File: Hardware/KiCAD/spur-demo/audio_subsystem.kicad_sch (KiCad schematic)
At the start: 25 parts, among them U3 MAX98357A, U4 LM393

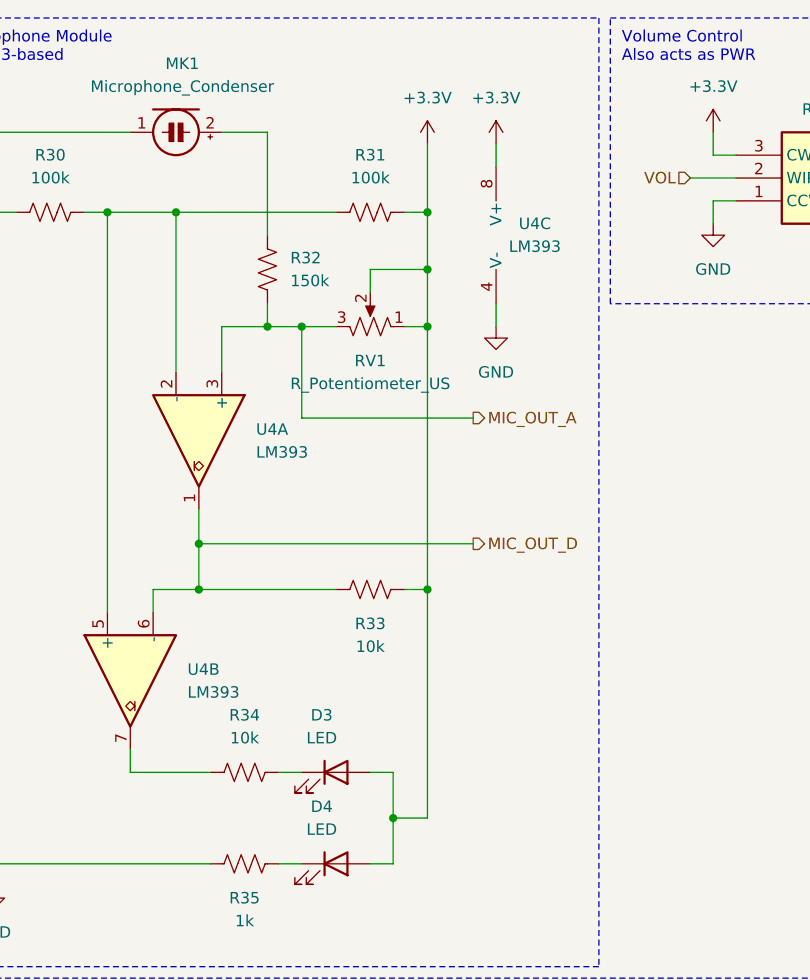
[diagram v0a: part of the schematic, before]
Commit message: fix: give mic level setpoint potentiometer a name
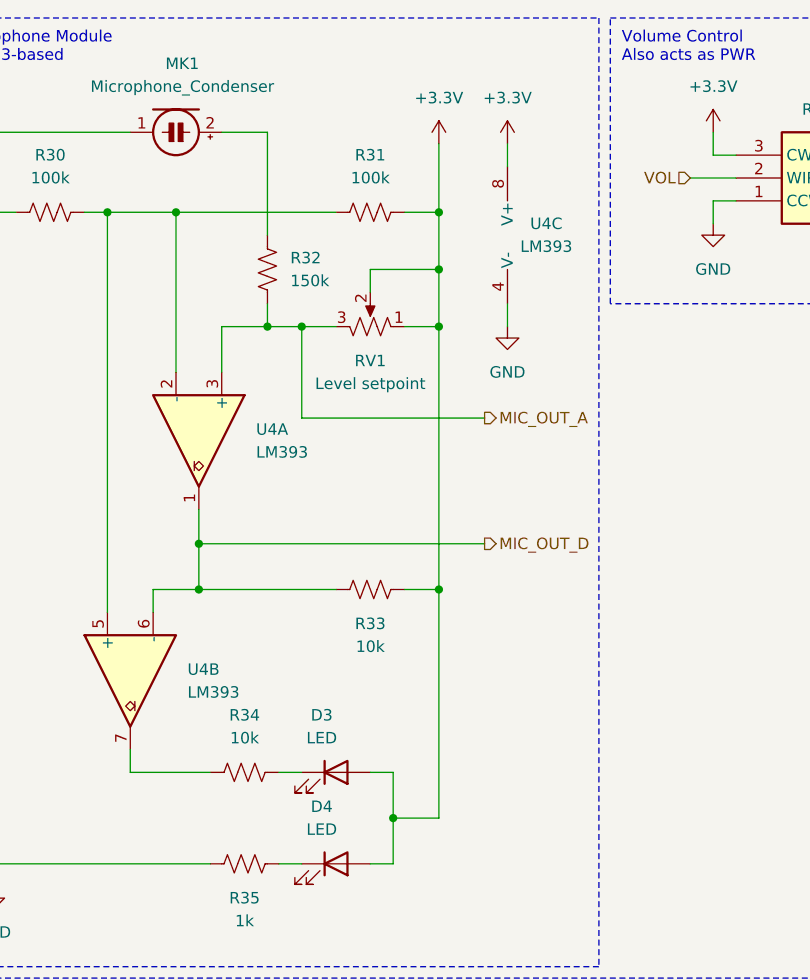
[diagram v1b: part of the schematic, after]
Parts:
- RV1: value R_Potentiometer_US -> Level setpoint
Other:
- moved on the sheet: U4C

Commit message: feat: begin footprint assignment, unify +3.3V PWRREFs
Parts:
- D3, D4: footprint (none) -> LED_SMD:LED_0603_1608Metric_Pad1.05x0.95mm_HandSolder
- LS1: footprint (none) -> Connector_JST:JST_XH_S2B-XH-A_1x02_P2.50mm_Horizontal
- MK1: footprint (none) -> Sensor_Audio:POM-2244P-C3310-2-R
- R13, R14, R28, R29, R30, R31, R32, R33, R34, R35, R37: footprint (none) -> Resistor_SMD:R_0603_1608Metric
- RV1: footprint (none) -> Potentiometer_SMD:Potentiometer_Bourns_3214W_Vertical
- U4: footprint (none) -> Package_SO:VSSOP-8_3x3mm_P0.65mm
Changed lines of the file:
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@@
 			)
 		)
-		(property "Footprint" ""
+		(property "Footprint" "LED_SMD:LED_0603_1608Metric_Pad1.05x0.95mm_HandSolder"
 			(at 57.15 107.95 0)
 			(effects
@@
 			)
 		)
-		(property "Footprint" ""
+		(property "Footprint" "LED_SMD:LED_0603_1608Metric_Pad1.05x0.95mm_HandSolder"
 			(at 57.15 97.79 0)
 			(effects
@@
 			)
 		)
-		(property "Footprint" ""
+		(property "Footprint" "Resistor_SMD:R_0603_1608Metric"
 			(at 46.736 98.806 90)
 			(effects
@@
 			)
 		)
-		(property "Footprint" ""
+		(property "Footprint" "Resistor_SMD:R_0603_1608Metric"
 			(at 249.174 100.076 90)
 			(effects
@@
 			)
 		)
-		(property "Footprint" ""
+		(property "Footprint" "Connector_JST:JST_XH_S2B-XH-A_1x02_P2.50mm_Horizontal"
 			(at 269.24 40.64 0)
 			(effects
@@
 			)
 		)
-		(property "Footprint" ""
+		(property "Footprint" "Package_SO:VSSOP-8_3x3mm_P0.65mm"
 			(at 41.91 60.96 0)
 			(effects
@@
 			)
 		)
-		(property "Footprint" ""
+		(property "Footprint" "Resistor_SMD:R_0603_1608Metric"
 			(at 60.706 36.576 90)
 			(effects
@@
 			)
 		)
-		(property "Footprint" ""
+		(property "Footprint" "Resistor_SMD:R_0603_1608Metric"
 			(at 46.736 108.966 90)
 			(effects
@@
 			)
 		)
-		(property "Footprint" ""
+		(property "Footprint" "Resistor_SMD:R_0603_1608Metric"
 			(at 60.706 78.486 90)
 			(effects
@@
 			)
 		)
-		(property "Footprint" ""
+		(property "Footprint" "Resistor_SMD:R_0603_1608Metric"
 			(at 228.346 84.836 90)
 			(effects
@@
 			)
 		)
-		(property "Footprint" ""
+		(property "Footprint" "Package_SO:VSSOP-8_3x3mm_P0.65mm"
 			(at 34.29 87.63 0)
 			(effects
@@
 			)
 		)
-		(property "Footprint" ""
+		(property "Footprint" "Resistor_SMD:R_0603_1608Metric"
 			(at 215.646 39.624 90)
 			(effects
@@
 			)
 		)
-		(property "Footprint" ""
+		(property "Footprint" "Resistor_SMD:R_0603_1608Metric"
 			(at 228.854 92.964 90)
 			(effects
@@
 			)
 		)
-		(property "Footprint" ""
+		(property "Footprint" "Package_SO:VSSOP-8_3x3mm_P0.65mm"
 			(at 78.74 38.1 0)
 			(effects
@@
 			)
 		)
-		(property "Footprint" ""
+		(property "Footprint" "Sensor_Audio:POM-2244P-C3310-2-R"
 			(at 41.91 26.67 90)
 			(effects
@@
 			)
 		)
-		(property "Footprint" ""
+		(property "Footprint" "Resistor_SMD:R_0603_1608Metric"
 			(at 25.146 36.576 90)
 			(effects
@@
 			)
 		)
-		(property "Footprint" ""
+		(property "Footprint" "Resistor_SMD:R_0603_1608Metric"
 			(at 225.044 146.304 90)
 			(effects
@@
 			)
 		)
-		(property "Footprint" ""
+		(property "Footprint" "Resistor_SMD:R_0603_1608Metric"
 			(at 50.546 42.164 90)
 			(effects
@@
 			)
 		)
-		(property "Footprint" ""
+		(property "Footprint" "Potentiometer_SMD:Potentiometer_Bourns_3214W_Vertical"
 			(at 60.96 48.26 0)
 			(effects

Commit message: feat: assign solder jumper footprints, begin testpoints
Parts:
- JP1, JP2: footprint (none) -> Jumper:SolderJumper-3_P1.3mm_Open_RoundedPad1.0x1.5mm_NumberLabels
- JP3, JP5: footprint (none) -> Jumper:SolderJumper-2_P1.3mm_Open_RoundedPad1.0x1.5mm
- JP4: footprint (none) -> Jumper:SolderJumper-2_P1.3mm_Bridged_Pad1.0x1.5mm
- JP6: footprint (none) -> Jumper:SolderJumper-3_P1.3mm_Bridged12_RoundedPad1.0x1.5mm_NumberLabels
- RV1: footprint Potentiometer_SMD:Potentiometer_Bourns_3214W_Vertical -> Potentiometer_SMD:Potentiometer_Bourns_3314G_Vertical
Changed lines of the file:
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@@
 			)
 		)
-		(property "Footprint" ""
+		(property "Footprint" "Jumper:SolderJumper-3_P1.3mm_Bridged12_RoundedPad1.0x1.5mm_NumberLabels"
 			(at 205.74 33.02 0)
 			(effects
@@
 			)
 		)
-		(property "Footprint" ""
+		(property "Footprint" "Jumper:SolderJumper-3_P1.3mm_Open_RoundedPad1.0x1.5mm_NumberLabels"
 			(at 212.09 147.32 0)
 			(effects
@@
 			)
 		)
-		(property "Footprint" ""
+		(property "Footprint" "Jumper:SolderJumper-2_P1.3mm_Bridged_Pad1.0x1.5mm"
 			(at 241.3 83.82 0)
 			(effects
@@
 			)
 		)
-		(property "Footprint" ""
+		(property "Footprint" "Jumper:SolderJumper-3_P1.3mm_Open_RoundedPad1.0x1.5mm_NumberLabels"
 			(at 231.14 139.7 0)
 			(effects
@@
 			)
 		)
-		(property "Footprint" ""
+		(property "Footprint" "Jumper:SolderJumper-2_P1.3mm_Open_RoundedPad1.0x1.5mm"
 			(at 241.3 73.66 0)
 			(effects
@@
 			)
 		)
-		(property "Footprint" ""
+		(property "Footprint" "Jumper:SolderJumper-2_P1.3mm_Open_RoundedPad1.0x1.5mm"
 			(at 241.3 93.98 0)
 			(effects
@@
 			)
 		)
-		(property "Footprint" "Potentiometer_SMD:Potentiometer_Bourns_3214W_Vertical"
+		(property "Footprint" "Potentiometer_SMD:Potentiometer_Bourns_3314G_Vertical"
 			(at 60.96 48.26 0)
 			(effects

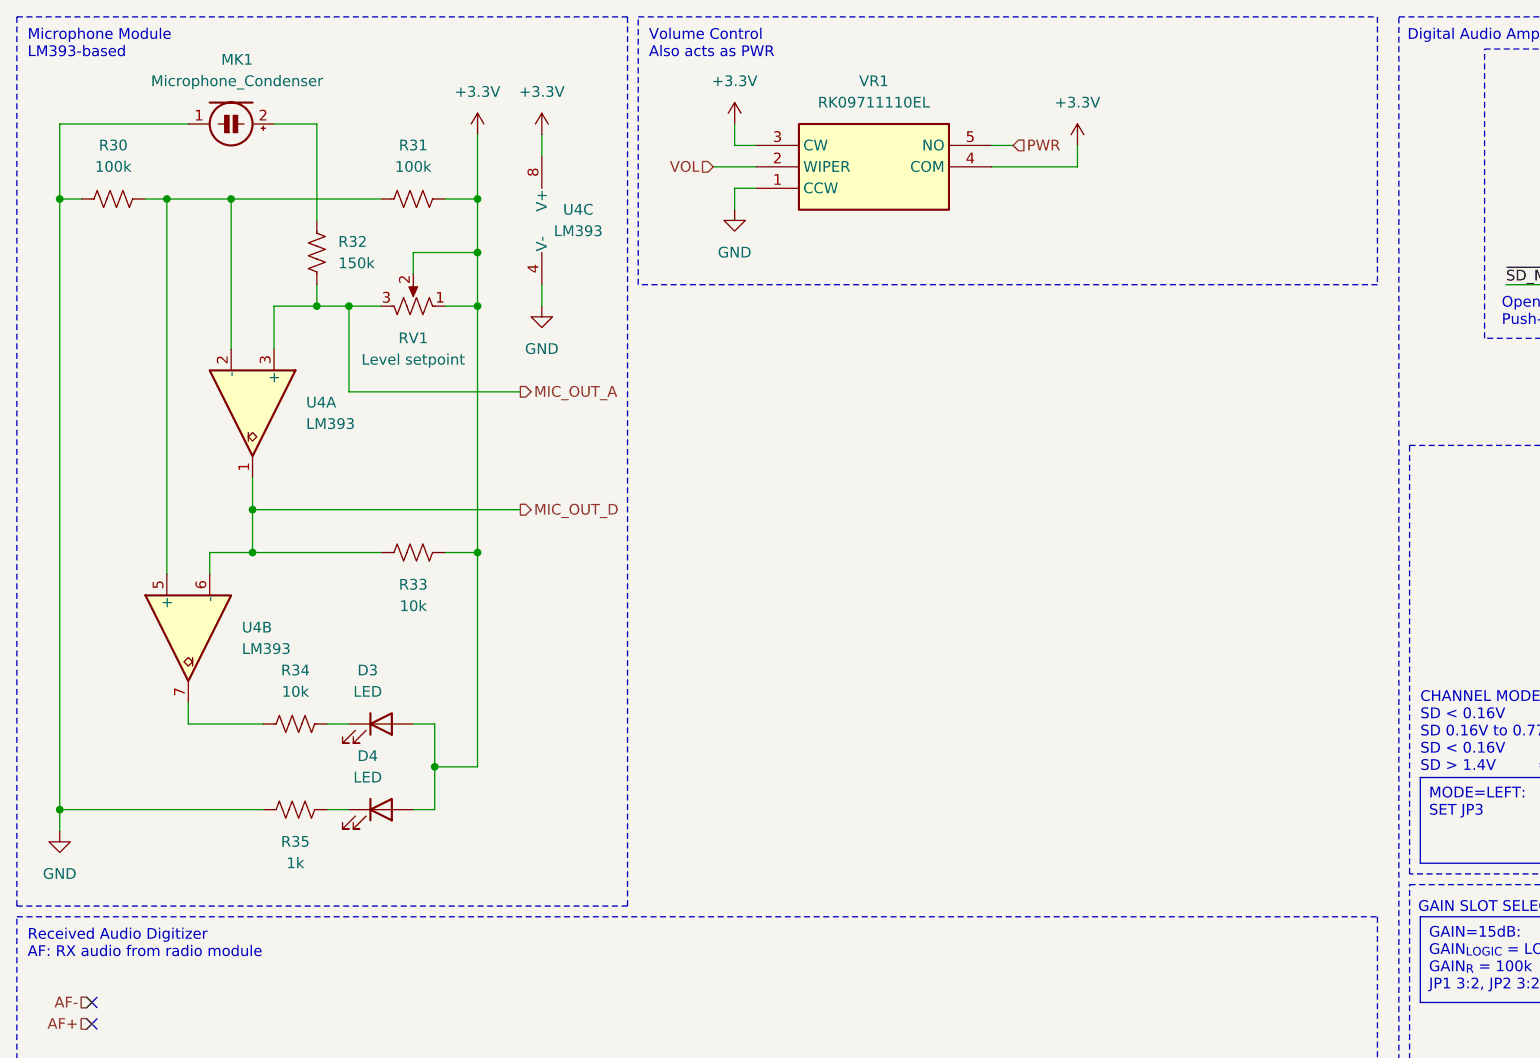
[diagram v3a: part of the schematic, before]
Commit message: feat: establish microphone module footprint and header
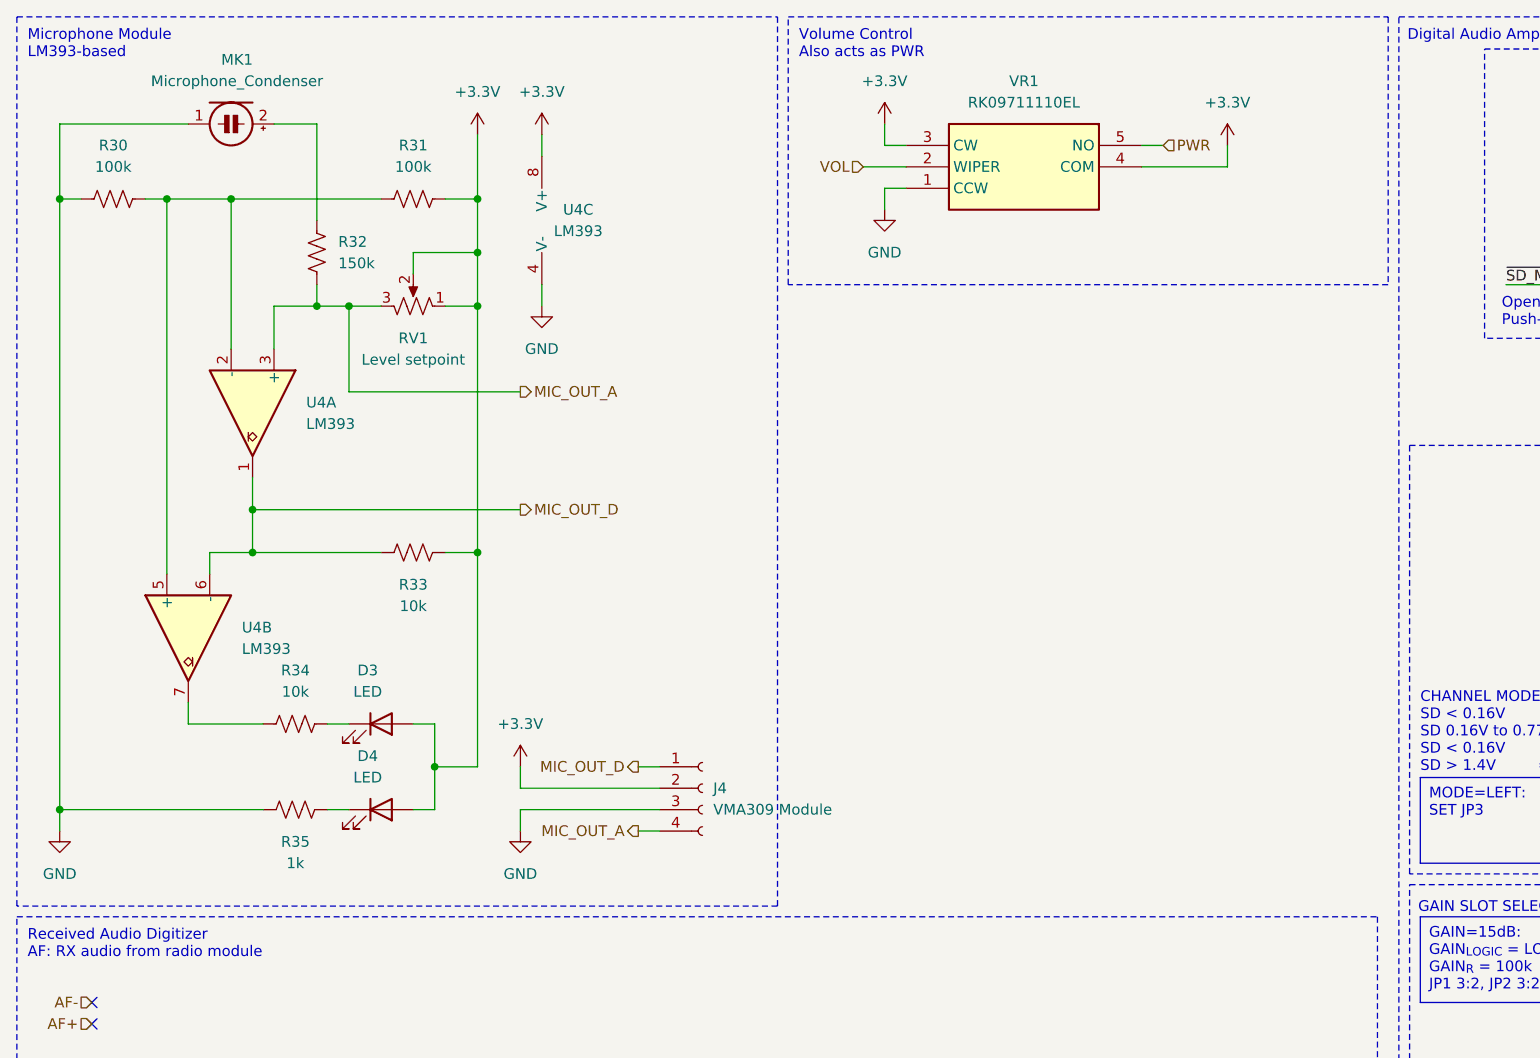
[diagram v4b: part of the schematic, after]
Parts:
- added J4: VMA309 Module, spur-demo:VMA309, symbol Connector:Conn_01x04_Socket
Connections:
- net +3.3V: now also J4.2 (Pin_2)
- net GND: now also J4.3 (Pin_3)
- net MIC_OUT_A: now also J4.4 (Pin_4)
- net MIC_OUT_D: now also J4.1 (Pin_1)
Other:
- moved on the sheet: VR1
